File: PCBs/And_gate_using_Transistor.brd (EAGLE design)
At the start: 17.3 x 30.2 mm, 8 parts, among them T1 BC547

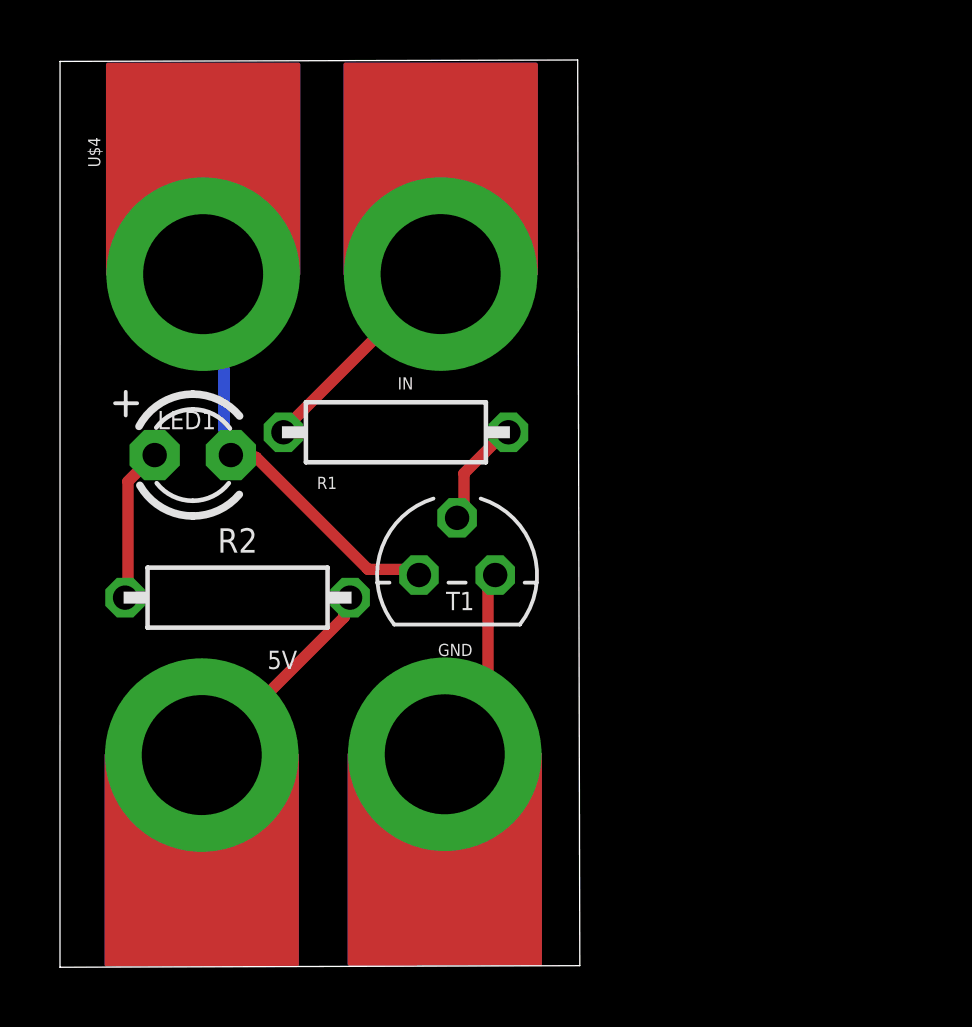
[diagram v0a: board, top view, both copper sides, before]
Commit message: Renamed files .
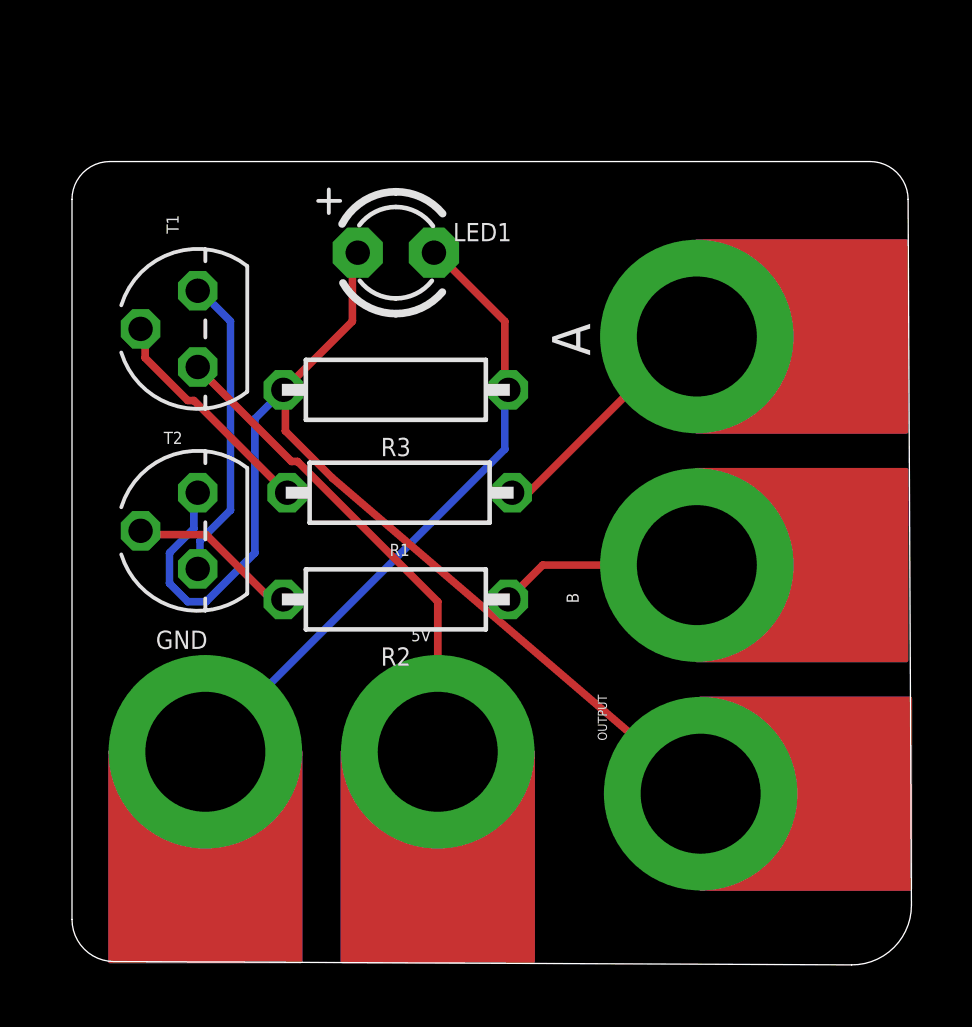
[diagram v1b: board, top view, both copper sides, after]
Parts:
- removed IN, U$4: MICROBIT_PAD, microbit:MICROBIT_PAD
- added A, B, OUTPUT: MICROBIT_PAD, microbit:MICROBIT_PAD
- added R3: (no value), we-rcl:R0207/7
- added T2: BC547, transistor-neu-to92:TO92
- R1: value 10k -> (none)
- R2: value 470 -> (none)
- T1: device transistor:TO92 -> transistor-neu-to92:TO92
- moved T1 11.9 mm to (4.19, 21.1), turned to 90 degrees
- moved LED1 9.56 mm to (10.8, 23.6)
- moved GND 7.98 mm to (4.45, 6.99)
- moved 5V 7.87 mm to (12.2, 6.99)
- moved R2 5.28 mm to (10.8, 12.1), turned to 180 degrees
- moved R1 2.02 mm to (10.9, 15.6), turned to 180 degrees
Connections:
- removed net N$4 (its old number): IN.PAD, R1.1
- removed net VOUT: LED1.K, T1.3, U$4.PAD
- new net N$1: R2.2, T2.2
- new net N$2: T1.1, T2.3
- new net N$6: A.PAD, R1.1
- new net N$7: B.PAD, R2.1
- net 5V: now also T1.3; no longer R2.2
- net GND: now also LED1.K, R3.1; no longer T1.1
- net N$3: now also OUTPUT.PAD, R3.2, T2.1; no longer R2.1
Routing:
- net N$3: track 5.16 -> 38.4 mm
- net GND: track 6.78 -> 21.9 mm
- net VOUT: track 14.4 -> 0.00 mm
- net N$2: track 0.00 -> 10.2 mm
- net 5V: track 7.40 -> 16.3 mm
- net N$6: track 0.00 -> 8.23 mm
- net N$4 (its old number): track 7.48 -> 0.00 mm
- net N$7: track 0.00 -> 6.76 mm
- net N$1: track 0.00 -> 5.70 mm
- net N$4: track 3.65 -> 7.62 mm
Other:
- board size 17.3 x 30.2 mm -> 28 x 26.8 mm
